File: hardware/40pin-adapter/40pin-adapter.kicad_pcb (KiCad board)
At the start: 2 copper layers, 16.1 x 51.5 mm, 3 parts, among them J1 Conn_02x20_Odd_Even, J2 Conn_02x20_Odd_Even

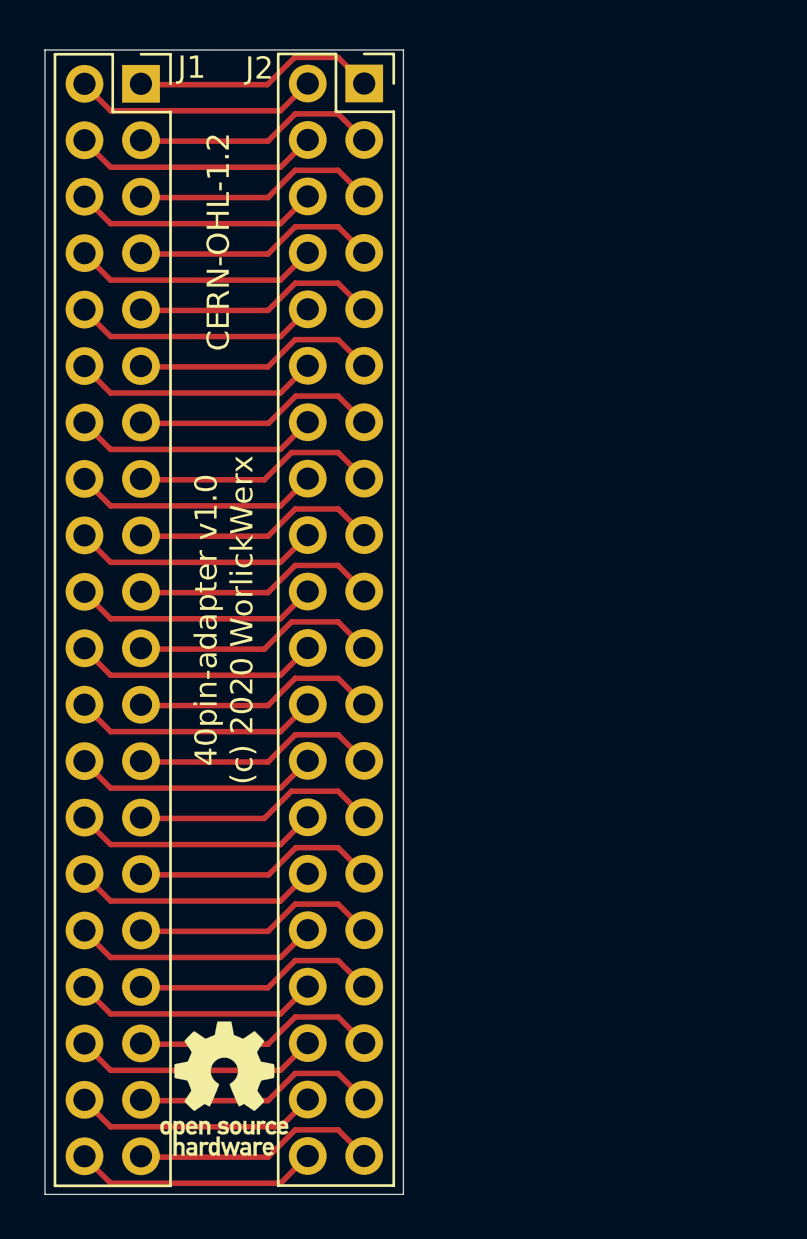
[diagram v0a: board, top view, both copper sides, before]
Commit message: hardware/40pin-adapter: use stackable connector
Rework this to use Samtec HLE-120-02-xxx-DV-BE-A
connector.  It is a low profile SMD connector with
holes to allow header pins to go through the board.

Call this version 2.0 on the silk screen.

Ordered from oshpark on 14 July 2020.
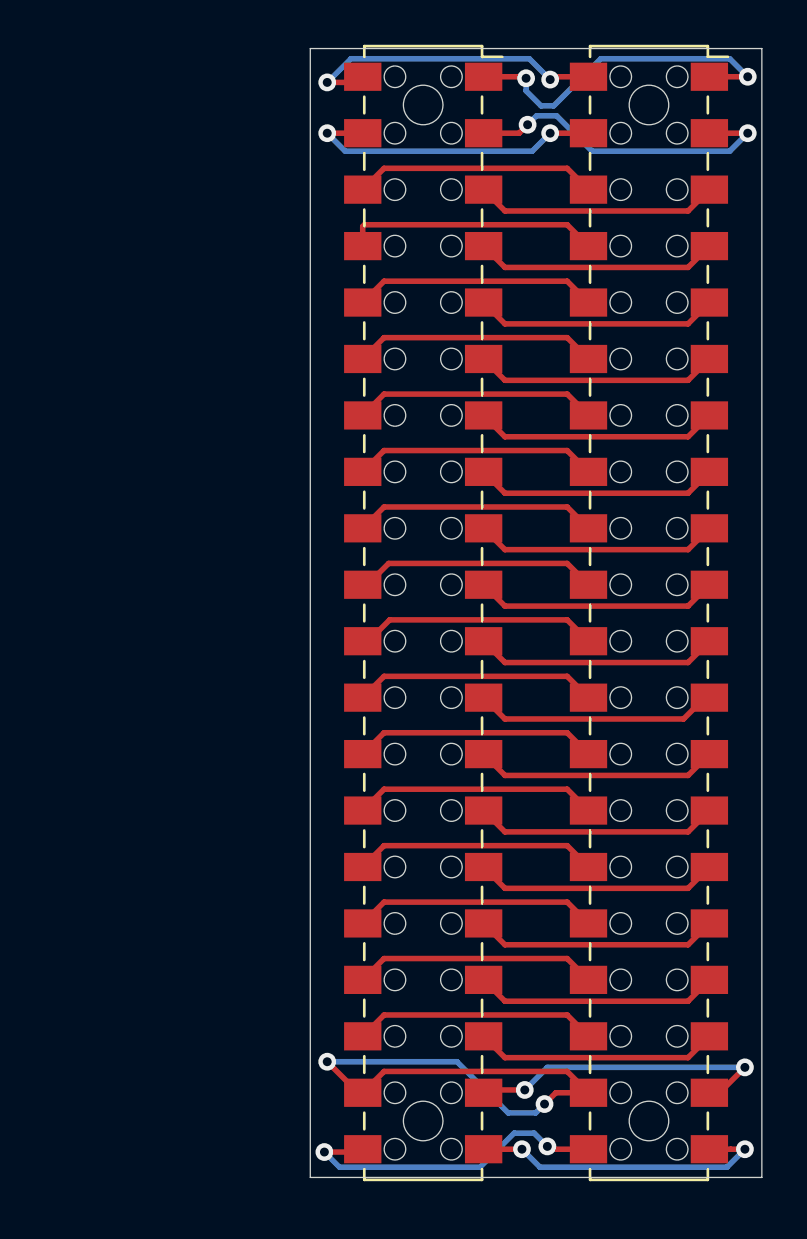
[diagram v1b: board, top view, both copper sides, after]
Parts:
- J1, J2: footprint Connector_PinSocket_2.54mm:PinSocket_2x20_P2.54mm_Vertical -> Connector_Samtec_HLE_SMD:Samtec_HLE-120-02-xxx-DV-BE-A_2x20_P2.54mm_Horizontal
- REF**: moved to B.Cu
- moved J2 27.1 mm to (165.1, 91.4), turned to 270 degrees
- moved J1 27.0 mm to (154.9, 91.4), turned to 270 degrees
- moved REF** 25.5 mm to (159.9, 91.4), turned to 90 degrees
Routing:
- net /PI38: track 11.0 -> 26.2 mm, vias 0 -> 2
- net /PI1: track 11.0 -> 15.7 mm, vias 0 -> 2
- net /PI3: track 11.0 -> 14.9 mm, vias 0 -> 2
- net /PI40: track 11.0 -> 14.9 mm, vias 0 -> 2
- net /PI2: track 11.0 -> 14.3 mm, vias 0 -> 2
- net /PI37: track 11.0 -> 14.3 mm, vias 0 -> 2
- net /PI39: track 11.0 -> 14.0 mm, vias 0 -> 2
- net /PI4: track 11.0 -> 14.0 mm, vias 0 -> 2
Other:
- board size 16.1 x 51.5 mm -> 20.3 x 50.8 mm
- board text added: "(c) WorlickWerx CERN-OHL-1.2"
- board text added: "1"
- board text added: "20pin-adapter v2.0"
- board text removed: "40pin-adapter v1.0 (c) 2020 WorlickWerx"
- board text removed: "CERN-OHL-1.2"
